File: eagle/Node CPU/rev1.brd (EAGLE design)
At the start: 100 x 86.3 mm, 22 parts, among them IC1 MEGA8-AI, Q1 8MHz

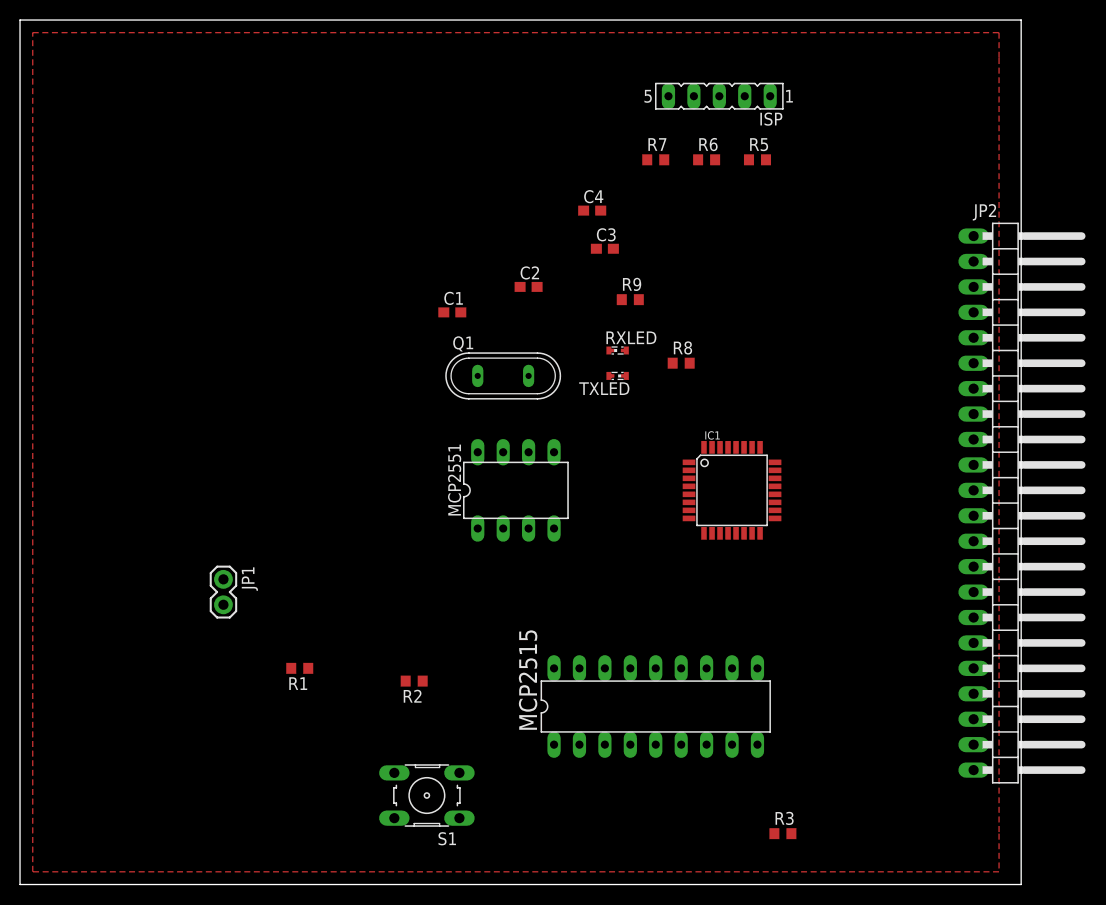
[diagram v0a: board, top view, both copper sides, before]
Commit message: finished rev 1 of node CPU board
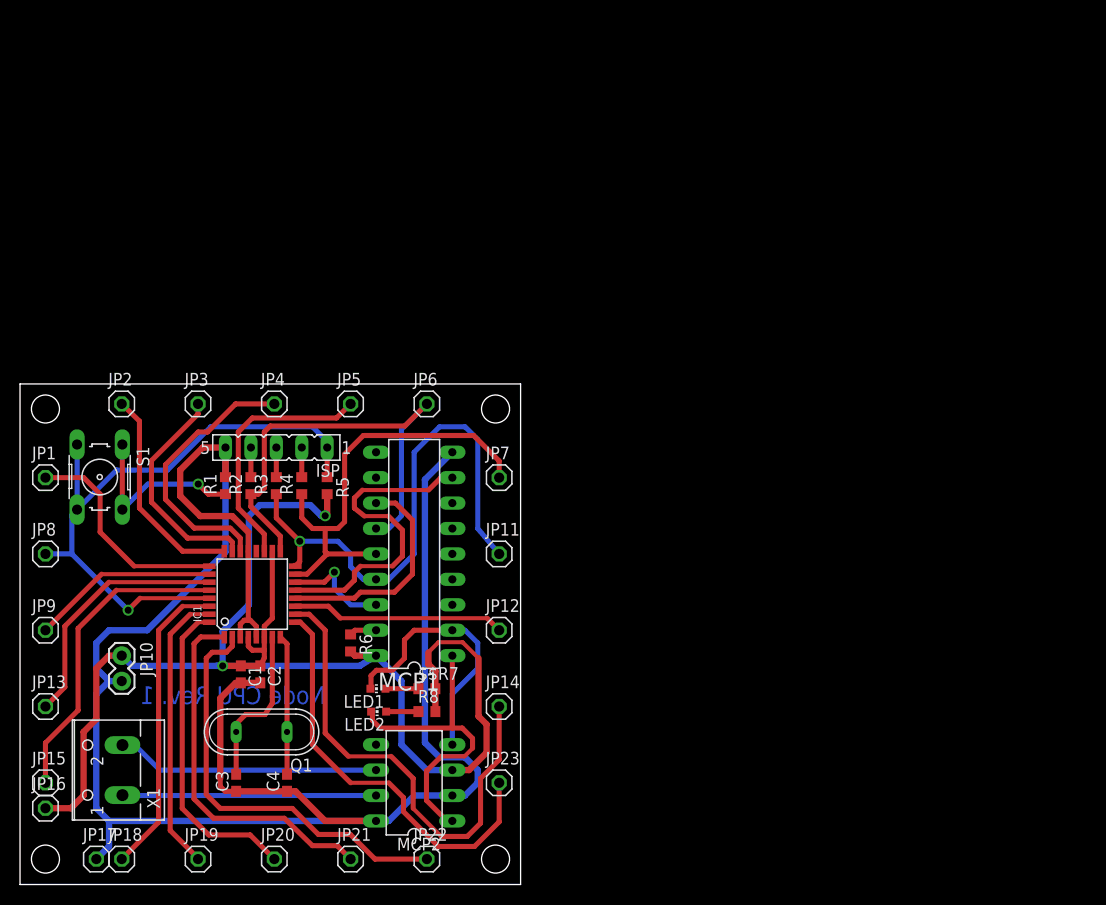
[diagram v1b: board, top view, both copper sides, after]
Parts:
- removed MCP2515: (no value), can:DIL18
- removed MCP2551: MCP2551DIL8, can:DIL08
- removed R7, R9: 470, resistor:R0603
- removed RXLED, TXLED: (no value), led:SMARTLED-TTW
- added $$R7, R4: 470, resistor:R0603
- added JP10: (no value), SparkFun-Passives:1X02
- added JP11, JP12, JP13, JP14, JP15, JP16, JP17, JP18, JP19, JP20, JP21, JP22, JP23, JP3, JP4, JP5, JP6, JP7, JP8, JP9: (no value), pinhead:1X01
- added LED1, LED2: (no value), led:CHIP-LED0603
- added MCP1: (no value), can:DIL18
- added MCP2: MCP2551DIL8, can:DIL08
- added X1: (no value), con-wago-500:W237-102
- C1: value 22pF -> 0.1uF
- C3: value 0.1uF -> 22pF
- JP1: device SparkFun-Passives:1X02 -> pinhead:1X01
- JP2: device pinhead:1X22/90 -> pinhead:1X01
- R1, R2: value 10K -> 470
- R5, R6: value 470 -> 10K
- moved JP2 89.5 mm to (10.2, 48.0), turned to 0 degrees
- moved C3 64.8 mm to (21.6, 10.2), turned to 90 degrees
- moved C4 64.8 mm to (26.7, 10.2), turned to 90 degrees
- moved R3 61.4 mm to (25.6, 39.8), turned to 90 degrees
- moved R6 59.9 mm to (33.0, 24.1), turned to 270 degrees
- moved ISP 56.5 mm to (25.6, 43.6)
- moved R5 53.9 mm to (30.7, 39.8), turned to 270 degrees
- moved IC1 49.0 mm to (23.2, 29.0), turned to 90 degrees
- moved C2 47.1 mm to (24.0, 21.0), turned to 270 degrees
- moved S1 45.6 mm to (7.96, 40.7), turned to 270 degrees
- moved R8 43.1 mm to (40.6, 17.3)
- moved Q1 43.0 mm to (24.1, 15.2), turned to 180 degrees
- moved C1 41.9 mm to (22.1, 21.0), turned to 270 degrees
- moved R2 25.4 mm to (23.1, 39.8), turned to 90 degrees
- moved JP1 20.5 mm to (2.54, 40.6), turned to 0 degrees
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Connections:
- removed net N$11: IC1.29, JP2.17, R1.1, S1.4
- removed net N$6: ISP.1
- removed net PC0: IC1.23, JP2.1
- removed net PC1: IC1.24, JP2.2
- removed net PC2: IC1.25, JP2.3
- removed net PC3: IC1.26, JP2.4
- removed net PC4: IC1.27, JP2.5
- removed net PC5: IC1.28, JP2.6
- removed net PC6: IC1.19, JP2.7
- removed net PC7: IC1.22, JP2.8
- removed net PD0: IC1.30, JP2.9
- removed net PD1: IC1.31, JP2.10
- removed net PD2: IC1.32, JP2.11
- removed net PD3: IC1.1, JP2.12
- removed net PD4: IC1.2, JP2.13
- removed net PD5: IC1.9, JP2.14
- removed net PD6: IC1.10, JP2.15
- removed net PD7: IC1.11, JP2.16
- new net N$20: IC1.23, JP3.1
- new net N$21: IC1.24, JP2.1
- new net N$22: IC1.25, JP1.1
- new net N$23: IC1.26, JP9.1
- new net N$24: IC1.27, JP13.1
- new net N$25: IC1.28, JP15.1
- new net N$26: IC1.19, JP5.1
- new net N$27: IC1.22, JP4.1
- new net N$28: IC1.30, JP18.1
- new net N$29: IC1.31, JP19.1
- new net N$30: IC1.32, JP20.1
- new net N$31: IC1.1, JP21.1
- new net N$32: IC1.2, JP22.1
- new net N$33: IC1.9, JP23.1
- new net N$34: IC1.10, JP14.1
- new net N$35: IC1.11, JP12.1
- new net N$36: MCP2.6, X1.2
- new net N$37: MCP2.7, X1.1
- new net RESET: IC1.29, ISP.1, JP8.1, R5.1, S1.3, S1.4
- net GND: now also C1.2, C2.2, C3.1, C4.1, JP10.2, JP17.1, MCP1.9, MCP2.2, MCP2.8, R1.2; no longer C1.1, C2.1, C3.2, C4.2, JP1.2, JP2.22, MCP2515.9, MCP2551.2, MCP2551.8, R3.2
- net N$1: now also JP6.1, MCP1.13, R2.1; no longer JP2.20, MCP2515.13, R7.1
- net N$10: now also C3.2; no longer C2.2
- net N$12: now also MCP1.17, R6.1; no longer MCP2515.17, R2.1
- net N$13: now also R1.1, S1.1; no longer R3.1
- net N$14: now also MCP1.12; no longer MCP2515.12
- net N$15: now also R4.2; no longer R5.2
- net N$16: now also R3.2; no longer R6.2
- net N$17: now also R2.2; no longer R7.2
- net N$18: now also LED2.A; no longer TXLED.A@1
- net N$19: now also $$R7.1, LED1.A; no longer R9.1, RXLED.A@1
- net N$2: now also JP11.1, MCP1.15, R3.1; no longer JP2.18, MCP2515.15, R6.1
- net N$3: now also JP7.1, MCP1.14, R4.1; no longer JP2.19, MCP2515.14, R5.1
- net N$4: now also MCP1.16; no longer MCP2515.16
- net N$5: now also MCP1.8; no longer MCP2515.8
- net N$7: now also LED2.C, MCP1.1, MCP2.1; no longer MCP2515.1, MCP2551.1, TXLED.C@1
- net N$9: now also C4.2; no longer C1.2
- net RXLED: now also LED1.C, MCP1.2, MCP2.4; no longer MCP2515.2, MCP2551.4, RXLED.C@1
- net VCC: now also $$R7.2, C1.1, C2.1, JP10.1, JP16.1, MCP1.18, MCP2.3, R5.2, R6.2; no longer C3.1, C4.1, JP1.1, JP2.21, MCP2515.18, MCP2551.3, R1.2, R2.2, R9.2
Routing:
- net GND: track 0.00 -> 191.7 mm
- net VCC: track 0.00 -> 137.5 mm, vias 0 -> 2
- net RESET: track 0.00 -> 63.1 mm, vias 0 -> 1
- net N$2: track 0.00 -> 53.7 mm, vias 0 -> 1
- net N$34: track 0.00 -> 48.5 mm
- net N$1: track 0.00 -> 46.8 mm
- net N$3: track 0.00 -> 44.8 mm
- net N$32: track 0.00 -> 42.3 mm
- net N$33: track 0.00 -> 41.8 mm
- net N$31: track 0.00 -> 37.0 mm
- net N$5: track 0.00 -> 32.5 mm
- net N$7: track 0.00 -> 31.8 mm
- net N$30: track 0.00 -> 31.7 mm
- net N$25: track 0.00 -> 31.5 mm
- net N$28: track 0.00 -> 30.4 mm
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- removed copper zone on layer 1, net GND
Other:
- board size 100 x 86.3 mm -> 50 x 50 mm
- board text added: "Node CPU Rev. 1"
